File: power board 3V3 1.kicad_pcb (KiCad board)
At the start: 2 copper layers, 25 parts, among them J1 Conn_02x15_Odd_Even, Q1 NMOS - HL3400A, Q2 PMOS - SI2301, Q3 PMOS - SI2301, U1 TP4056-42-ESOP8, U2 HT7533-1-SOT89, U3 LM358DR

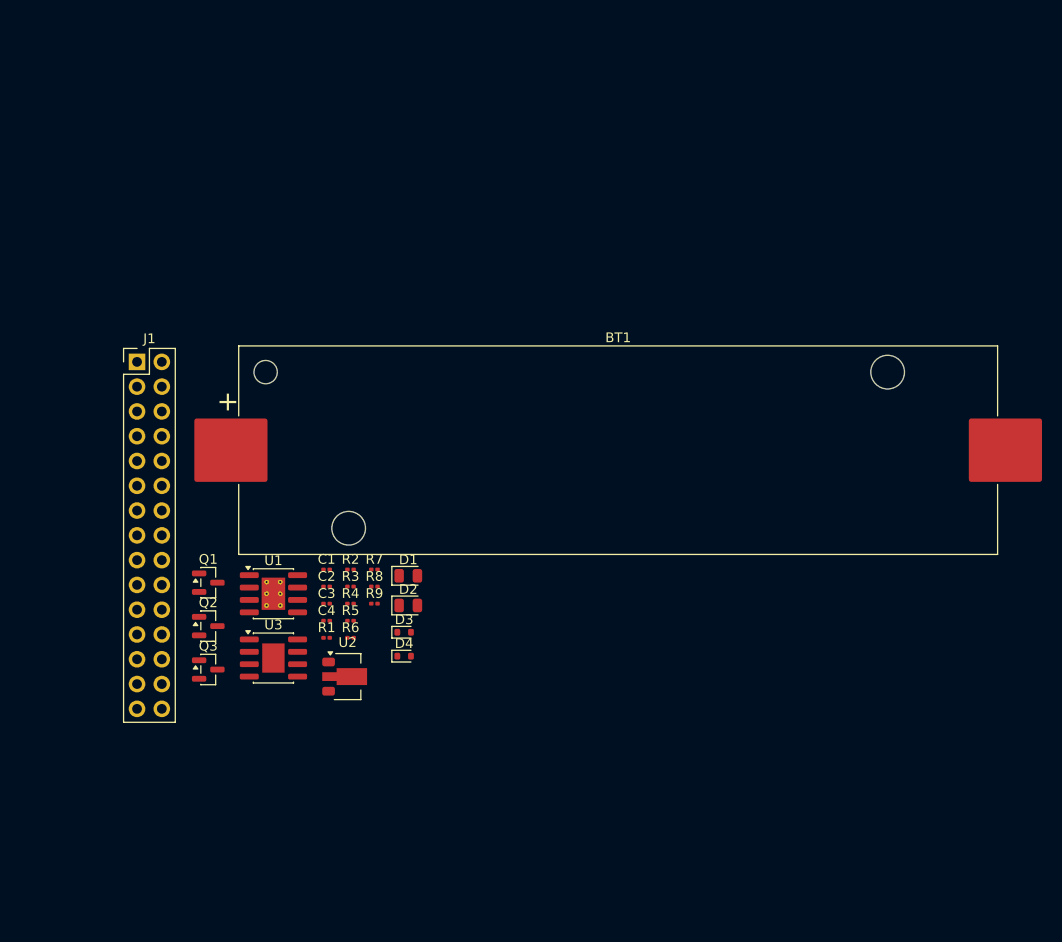
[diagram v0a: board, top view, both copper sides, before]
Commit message: Next is just silk screen labelling and ask Si Teng if Im retarded
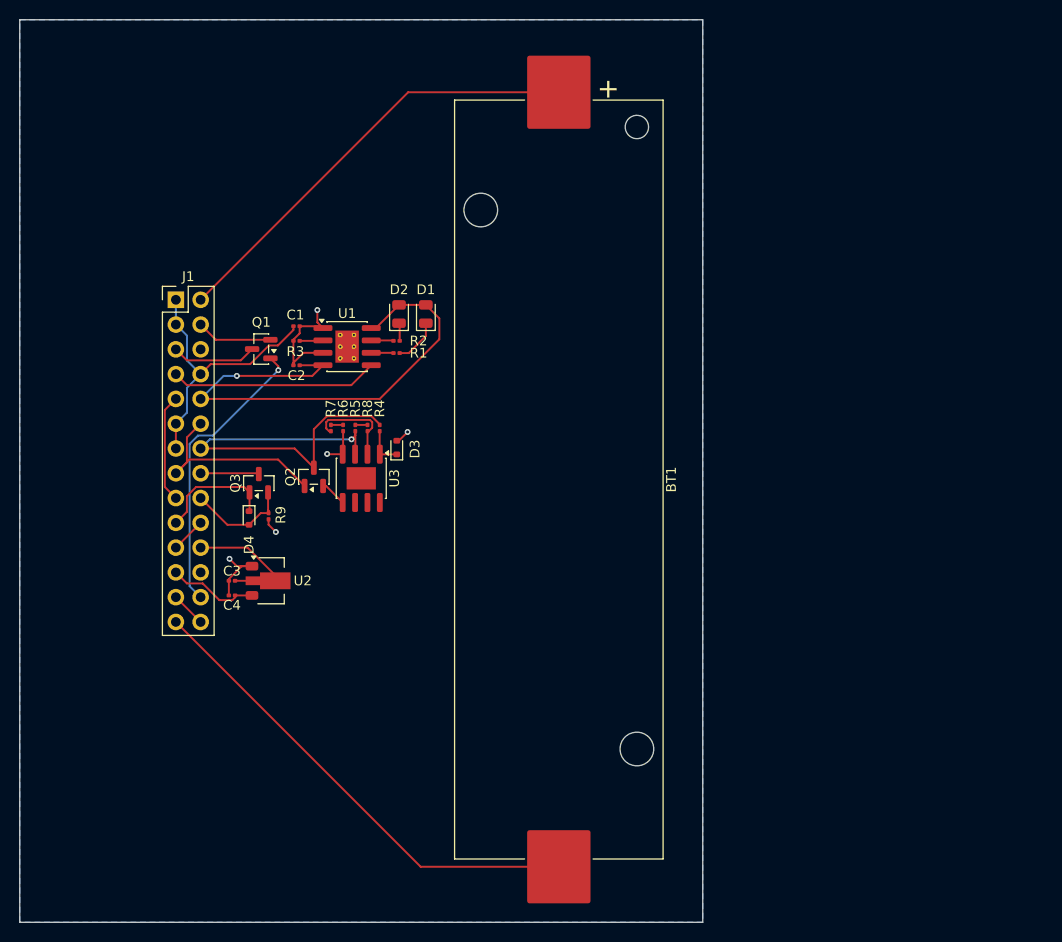
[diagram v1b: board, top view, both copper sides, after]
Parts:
- J1: value Conn_02x15_Odd_Even -> Conn_02x14_Odd_Even; footprint Connector_PinHeader_2.54mm:PinHeader_2x15_P2.54mm_Vertical -> Connector_PinHeader_2.54mm:PinHeader_2x14_P2.54mm_Vertical
- moved R1 30.1 mm to (161.1, 76.7)
- moved D2 29.9 mm to (161.4, 72.7), turned to 90 degrees
- moved D1 26.9 mm to (164.1, 72.7), turned to 90 degrees
- moved U1 26.4 mm to (156.1, 76.0)
- moved R3 25.8 mm to (150.9, 75.4), turned to 180 degrees
- moved C1 25.1 mm to (150.9, 73.9)
- moved Q1 24.6 mm to (147.2, 76.2), turned to 180 degrees
- moved R2 23.9 mm to (161.1, 75.4)
- moved C2 22.9 mm to (150.9, 77.9), turned to 180 degrees
- moved R6 21.5 mm to (155.6, 84.3), turned to -90 degrees
- moved D4 21.3 mm to (146.0, 93.6), turned to -90 degrees
- moved U3 20.5 mm to (157.5, 89.5), turned to -90 degrees
- moved Q3 19.8 mm to (147.0, 90.0), turned to 90 degrees
- moved R5 19.8 mm to (156.9, 84.3), turned to 90 degrees
- moved D3 18.9 mm to (161.1, 86.3), turned to 90 degrees
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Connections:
- BT1 pad 1: /FUSE2 -> /+BATT2
- J1 pad 10: /+BATT2 -> /POW CHRGR2
- J1 pad 11: /-BATT1 -> +BATT
- J1 pad 12: -BATT -> /+BATT_UVLO
- J1 pad 14: /+RPP2 -> /UVLO ON2
- J1 pad 15: -BATT -> /+BATT_UVLO
- J1 pad 16: /-RPP2 -> /UVLO2SEL2
- J1 pad 17: /RPPGND1 -> +5V
- J1 pad 18: GND -> /USB2SEL2
- J1 pad 19: /SELECTOR OUT2 -> /SELECTOR OUT1
- J1 pad 2: /+BATT_UVLO -> /+BATT2
- J1 pad 20: /VREG2 -> /SELECTOR OUT2
- J1 pad 21: /VREGOUT1 -> /SELECTOR OUT2
- J1 pad 22: +3V3 -> /VREG2
- J1 pad 23: +5V -> /VREGOUT1
- J1 pad 24: /USB2SEL2 -> +3V3
- J1 pad 25: /+BATT_UVLO -> -BATT
- J1 pad 26: /UVLO2SEL2 -> /-RPP2
- J1 pad 27: /SELECTOR OUT1 -> /-BATT1
- J1 pad 28: /SELECTOR OUT2 -> -BATT
- J1 pad 4: /UVLO ON2 -> /+RPP2
- J1 pad 5: +5V -> /RPPGND1
- J1 pad 6: /POW CHRGR2 -> GND
- J1 pad 9: +BATT -> +5V
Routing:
- net /POW CHRGR2: track 0.00 -> 54.0 mm, vias 0 -> 1
- net /-BATT1: track 0.00 -> 49.6 mm
- net /+BATT2: track 0.00 -> 45.5 mm
- net /UVLO ON2: track 0.00 -> 43.3 mm, vias 0 -> 1
- net /-RPP2: track 0.00 -> 30.0 mm, vias 0 -> 1
- net +BATT: track 0.00 -> 29.1 mm
- net GND: track 0.00 -> 26.8 mm, vias 0 -> 5
- net /BATT2CHRG1: track 0.00 -> 21.3 mm
- net /+BATT_UVLO: track 0.00 -> 21.0 mm
- net /VREG2: track 0.00 -> 14.3 mm
- net /SELECTOR OUT1: track 0.00 -> 12.2 mm
- net +5V: track 0.00 -> 11.1 mm
- net /USB2SEL2: track 0.00 -> 10.7 mm
- net /Vtest: track 0.00 -> 9.71 mm
- net /VREGOUT1: track 0.00 -> 9.29 mm
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- added copper zone on B.Cu, net GND
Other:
- board outline added: 70 x 92.5 mm
